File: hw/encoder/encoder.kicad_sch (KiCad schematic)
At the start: 1 part, among them U2 AS5147-TS_EK_AB

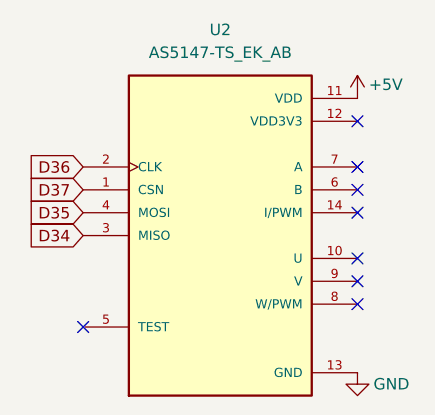
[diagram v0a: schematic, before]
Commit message: update schematics
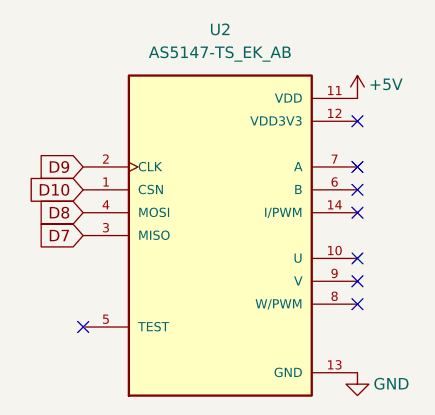
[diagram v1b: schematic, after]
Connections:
- net D34 renamed D7
- net D35 renamed D8
- net D36 renamed D9
- net D37 renamed D10
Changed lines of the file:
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@@
 		(at 149.86 83.82)
 	)
-	(global_label "D37"
+	(global_label "D10"
 		(shape input)
 		(at 119.38 83.82 180)
@@
 		)
 	)
-	(global_label "D36"
+	(global_label "D9"
 		(shape input)
 		(at 119.38 81.28 180)
@@
 		)
 		(property "Intersheetrefs" "${INTERSHEET_REFS}"
-			(at 112.7058 81.28 0)
+			(at 113.9153 81.28 0)
 			(hide yes)
 			(show_name no)
@@
 		)
 	)
-	(global_label "D35"
+	(global_label "D8"
 		(shape input)
 		(at 119.38 86.36 180)
@@
 		)
 		(property "Intersheetrefs" "${INTERSHEET_REFS}"
-			(at 112.7058 86.36 0)
+			(at 113.9153 86.36 0)
 			(hide yes)
 			(show_name no)
@@
 		)
 	)
-	(global_label "D34"
+	(global_label "D7"
 		(shape input)
 		(at 119.38 88.9 180)
@@
 		)
 		(property "Intersheetrefs" "${INTERSHEET_REFS}"
-			(at 112.7058 88.9 0)
+			(at 113.9153 88.9 0)
 			(hide yes)
 			(show_name no)
